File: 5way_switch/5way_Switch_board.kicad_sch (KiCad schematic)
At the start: 6 parts, among them J1 CONN_01X8, SW1 5way-switch

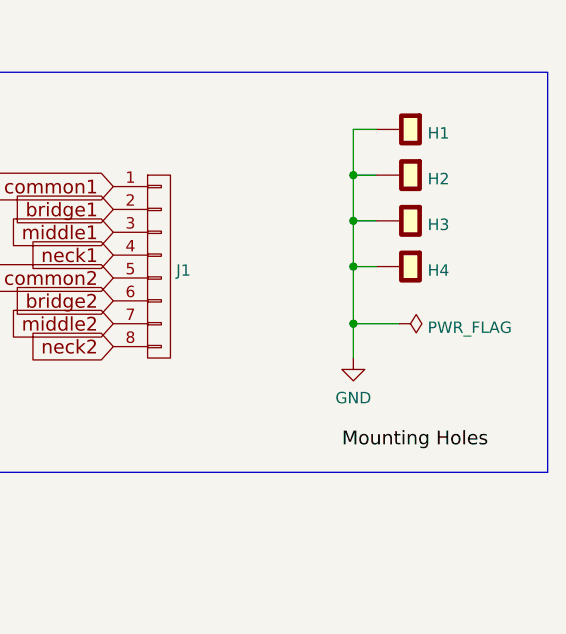
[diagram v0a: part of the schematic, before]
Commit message: More updates. I think we're good.
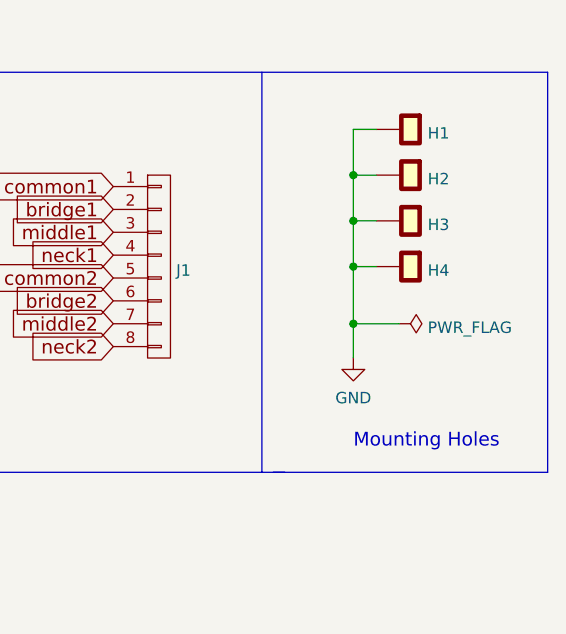
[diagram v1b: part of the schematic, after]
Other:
- note added: "Mounting Holes"
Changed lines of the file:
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@@
+    (stroke (width 0) (type default) (color 0 0 0 0))
+  )
+  (polyline (pts (xy 189.23 100.33) (xy 190.5 100.33))
     (stroke (width 0) (type default) (color 0 0 0 0))
   )
@@
     (stroke (width 0) (type default) (color 0 0 0 0))
   )
+  (polyline (pts (xy 187.96 55.88) (xy 187.96 100.33))
+    (stroke (width 0) (type default) (color 0 0 0 0))
+  )
   (wire (pts (xy 198.12 72.39) (xy 200.66 72.39))
     (stroke (width 0) (type default) (color 0 0 0 0))
@@
     (effects (font (size 1.524 1.524)) (justify left bottom))
   )
-  (label "Mounting Holes" (at 196.85 97.79 0)
+  (text "Mounting Holes" (at 198.12 97.79 0)
     (effects (font (size 1.524 1.524)) (justify left bottom))
   )
